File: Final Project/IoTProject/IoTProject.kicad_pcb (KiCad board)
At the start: 2 copper layers, 1 part, among them IC1 STM32WB55CEU6

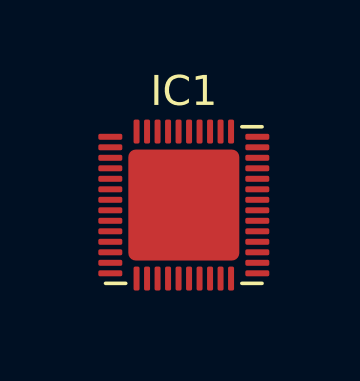
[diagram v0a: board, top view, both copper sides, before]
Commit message: More final report
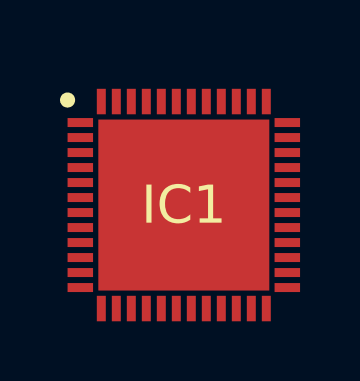
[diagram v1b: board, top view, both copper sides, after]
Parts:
- IC1: footprint Package_DFN_QFN:QFN-48-1EP_5x5mm_P0.35mm_EP3.7x3.7mm -> STM32WB55CEU6:QFN50P700X700X65-49N-D
